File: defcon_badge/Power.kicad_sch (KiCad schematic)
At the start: 15 parts, among them J10 USB_C_Receptacle_USB2.0_16P, J11 JST-PH 2P, SW1 SS-12D00, U10 TP4056, U11 ME6211C33M5G

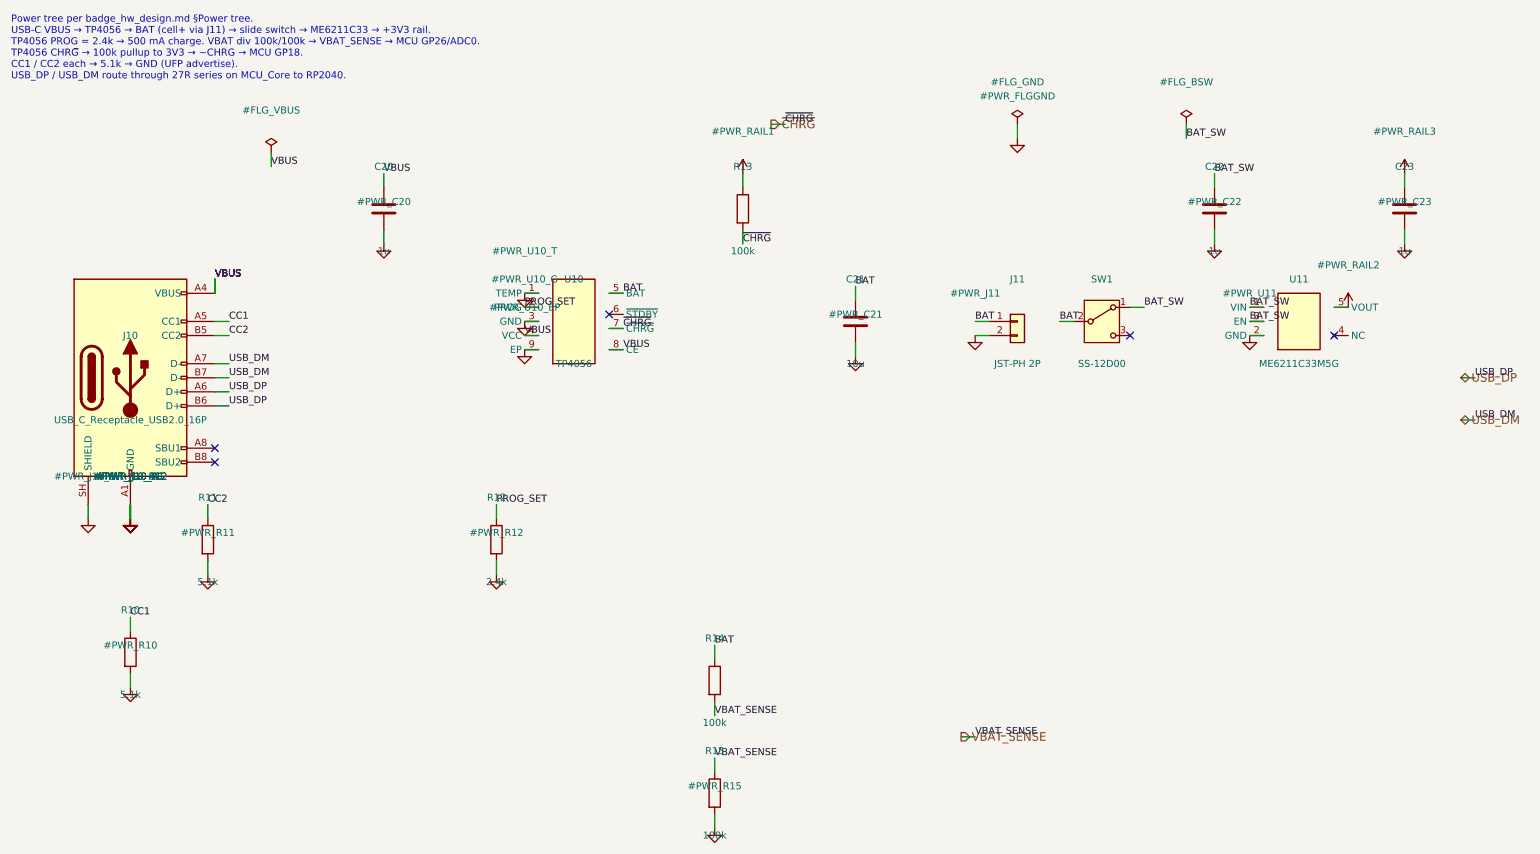
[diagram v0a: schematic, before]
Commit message: Routing redo
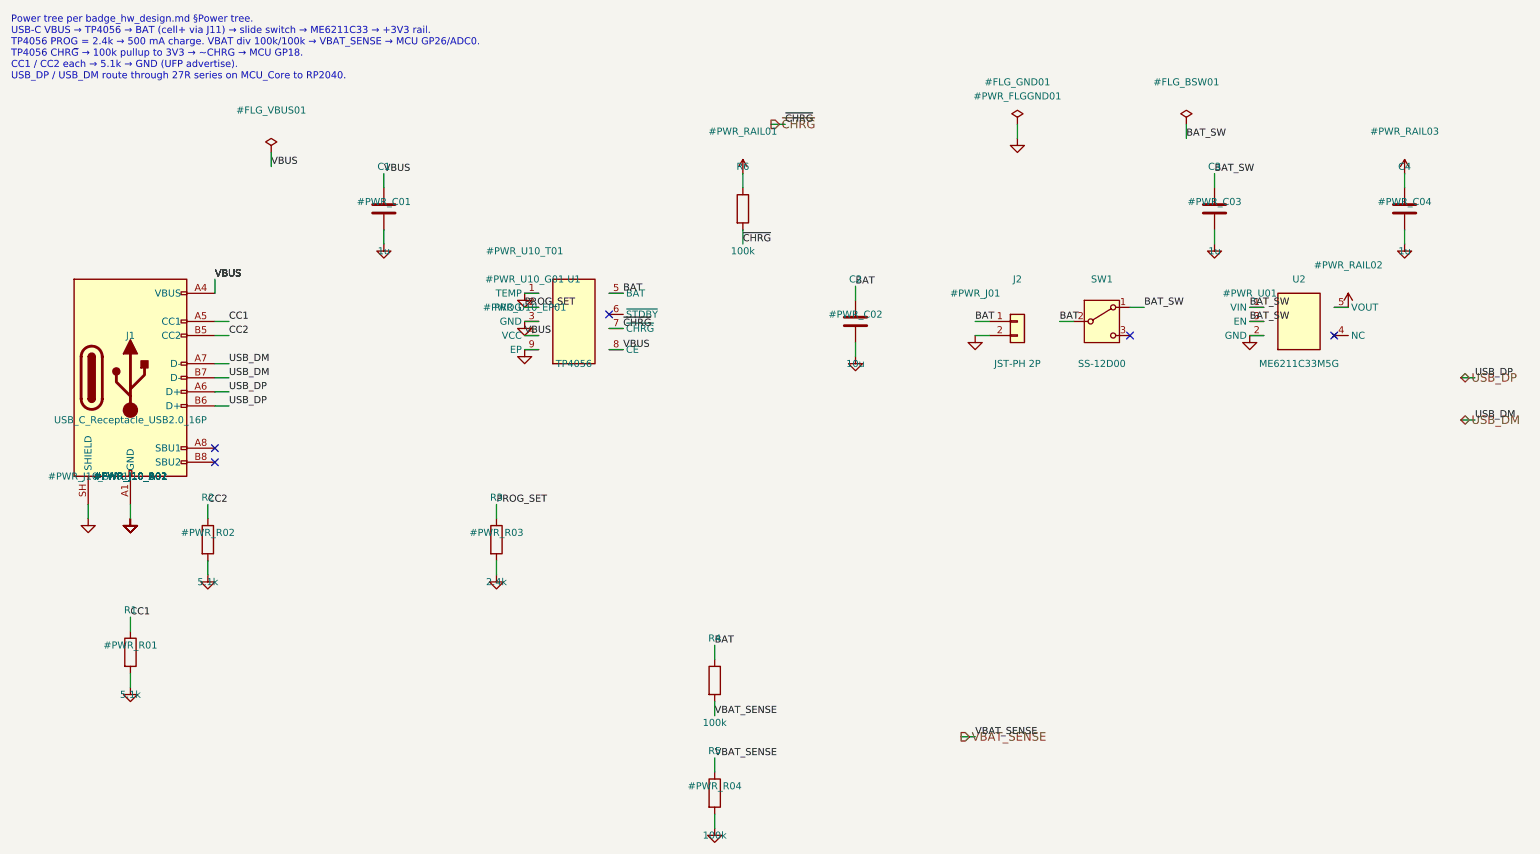
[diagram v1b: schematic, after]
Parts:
- renumbered C20 to C1, C21 to C2, C22 to C3, C23 to C4, J10 to J1, J11 to J2, R10 to R1, R11 to R2, R12 to R3, R14 to R4, R15 to R5, R13 to R6, U10 to U1, U11 to U2
